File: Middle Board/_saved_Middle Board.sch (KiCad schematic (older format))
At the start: 55 parts, among them J1 JTAG Connector, J2 Conn_Coaxial, J3 Conn_Coaxial, SW1 SW_SPST, U1 ATSAMG55, U2 BNO055_Breakout, U3 MS5803, U4 PD0810J5050S2HF, U5 XBee_PRO_SX

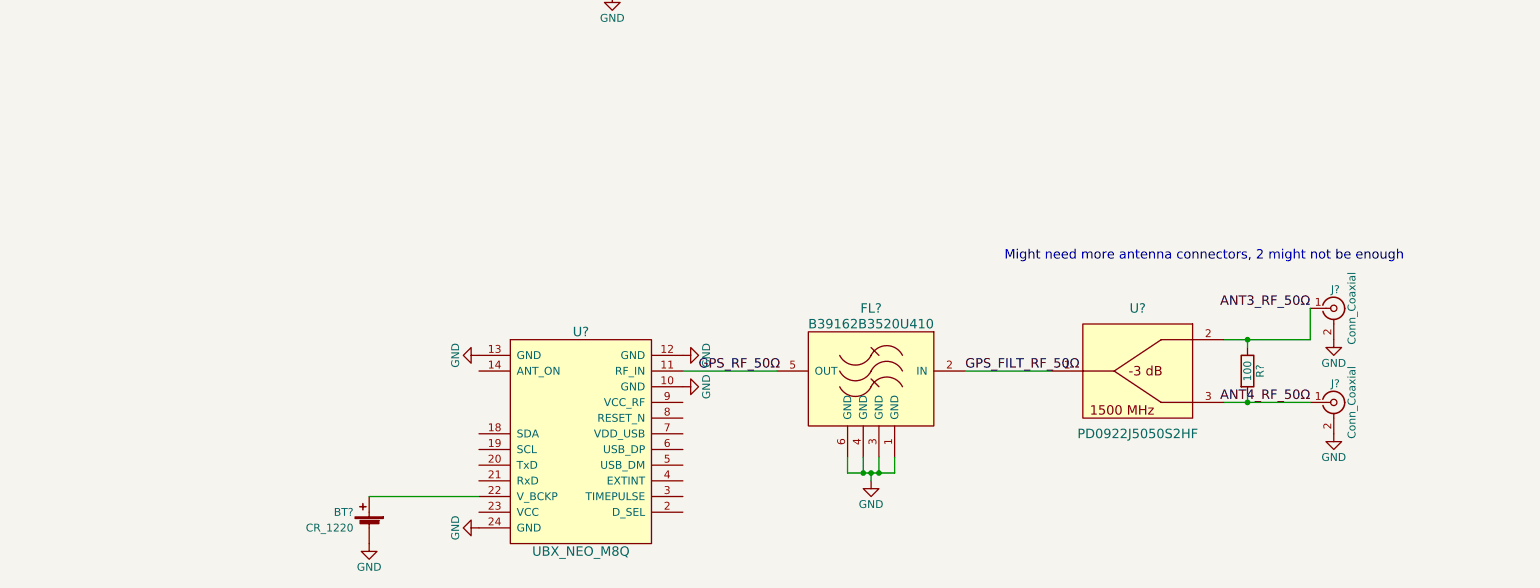
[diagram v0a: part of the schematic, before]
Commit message: Small changes
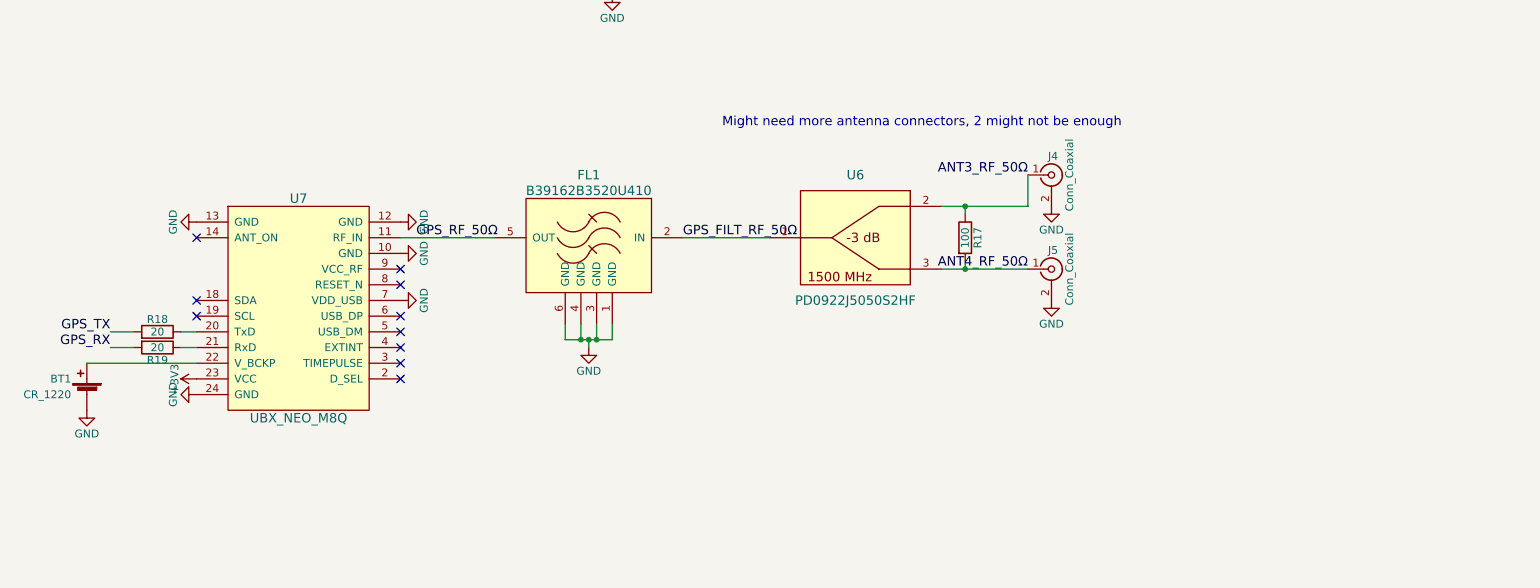
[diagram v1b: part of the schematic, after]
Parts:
- added R18, R19: 20, symbol R
- gave numbers to parts that had none: 7
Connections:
- net +3V3: now also U7.23 (VCC)
- net GND: now also U7.7 (VDD_USB)
- net at U7.20 (TxD): now also R18.1
- net at U7.21 (RxD): now also R19.1
- new net GPS_RX: R19.2
- new net GPS_TX: R18.2
- no-connect marks 24 -> 34
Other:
- moved on the sheet: BT1, FL1, J4, J5, R17, U6, U7
